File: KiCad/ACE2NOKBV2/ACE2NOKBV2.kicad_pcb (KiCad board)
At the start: 2 copper layers, 160 x 100 mm, 105 parts, among them IC1 78T, IC2 74367N, Q1 2N3904, Q2 2N3904, Q3 BC237, X1 6.556MHz

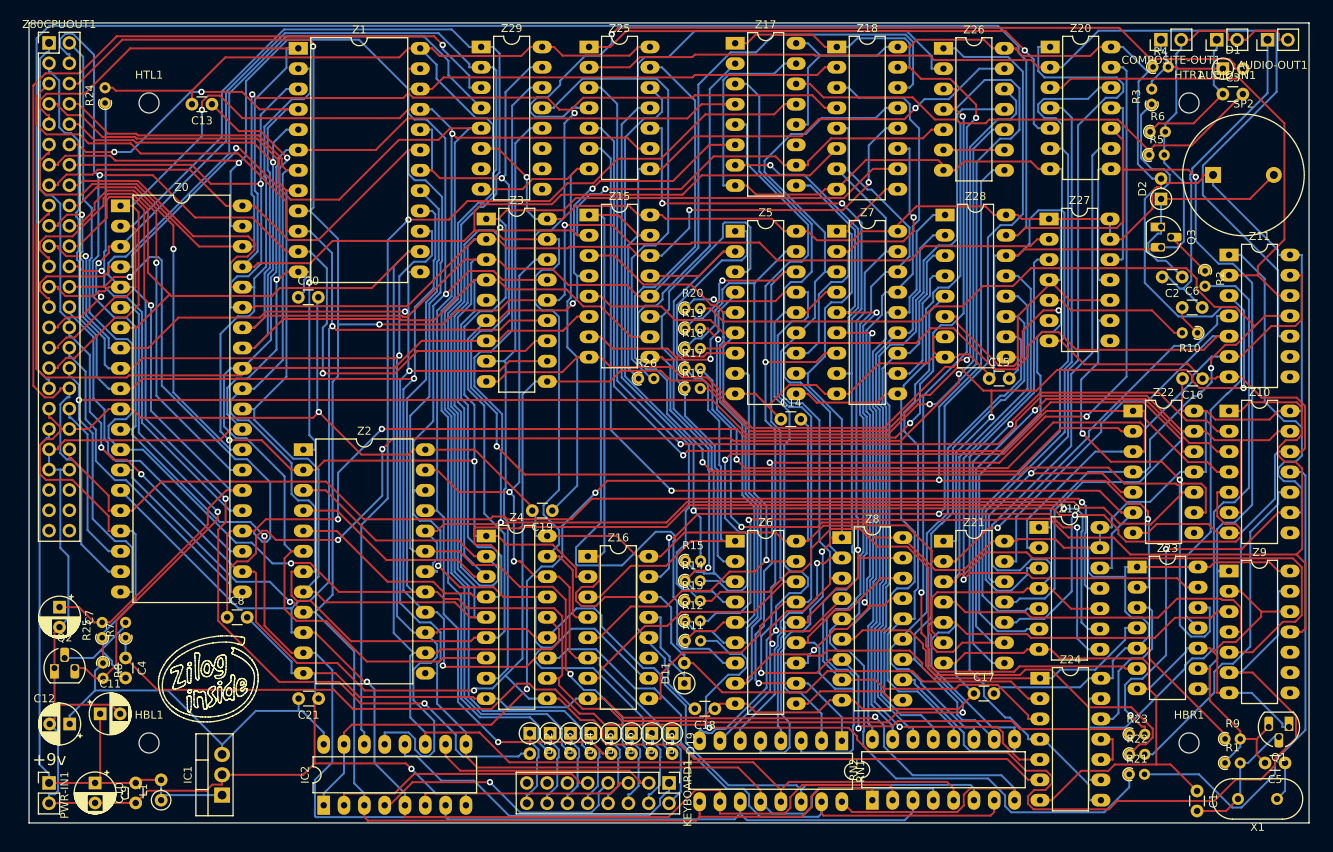
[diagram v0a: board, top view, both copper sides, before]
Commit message: Improve consitancy.
Signed-off-by: John Bradley <flypie@rocketmail.com>
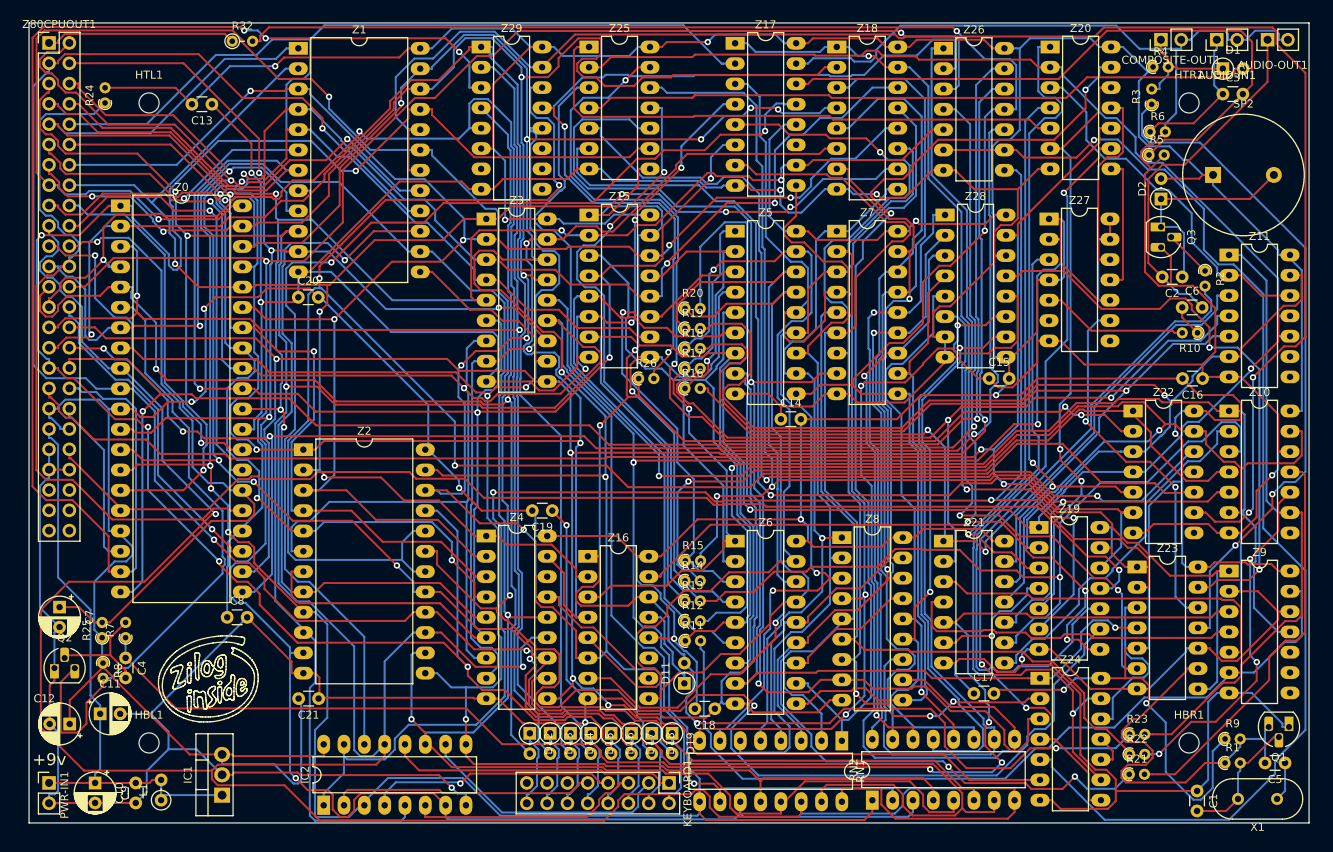
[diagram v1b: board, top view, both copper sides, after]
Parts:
- added R32: 1K0, Resistor_THT:R_Axial_DIN0204_L3.6mm_D1.6mm_P2.54mm_Vertical, F.Cu at (96.5, 41.7)
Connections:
- Z26 pad 11: /#WE -> Net-(R32-Pad2)
- Z5 pad 10: /#WE -> Net-(R32-Pad2)
- Z6 pad 10: /#WE -> Net-(R32-Pad2)
- Z7 pad 10: /#WE -> Net-(R32-Pad2)
- Z8 pad 10: /#WE -> Net-(R32-Pad2)
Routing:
- net Net-(R32-Pad2): track 0.00 -> 222.2 mm, vias 0 -> 2
- net /DA5: track 235.2 -> 377.6 mm, vias 2 -> 3
- net #NMI: track 777.6 -> 907.2 mm, vias 2 -> 13
- net /#WE: track 117.0 -> 23.9 mm
- net GND: track 839.2 -> 928.6 mm, vias 3 -> 9
- net #CPUCLK: track 305.9 -> 229.7 mm, vias 1 -> 2
- net /DA1: track 257.0 -> 330.8 mm, vias 2 -> 5
- net Net-(Z2-Pad18): track 169.2 -> 239.6 mm, vias 1 -> 3
- net /A10: track 257.5 -> 319.8 mm, vias 2 -> 4
- net /DA6: track 232.9 -> 277.7 mm, vias 2 -> 3
- net Net-(Z24-Pad5): track 109.0 -> 151.5 mm
- net /A11: track 203.4 -> 244.3 mm, vias 3 -> 5
- net /A8: track 246.9 -> 285.2 mm, vias 4 -> 8
- net Net-(Z1-Pad18): track 169.7 -> 206.9 mm
- net /A4: track 257.5 -> 220.8 mm, vias 2 -> 5
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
